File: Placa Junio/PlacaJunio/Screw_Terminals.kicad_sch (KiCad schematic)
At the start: 16 parts, among them J3 Terminal Paracaidas 2, J4 Terminal Paracaidas 1, J5 Terminal Paracaidas 3, J6 Terminal Paracaidas 4, Q2 IRLML0030, Q3 IRLML0030, Q5 IRLML0030, Q6 IRLML0030

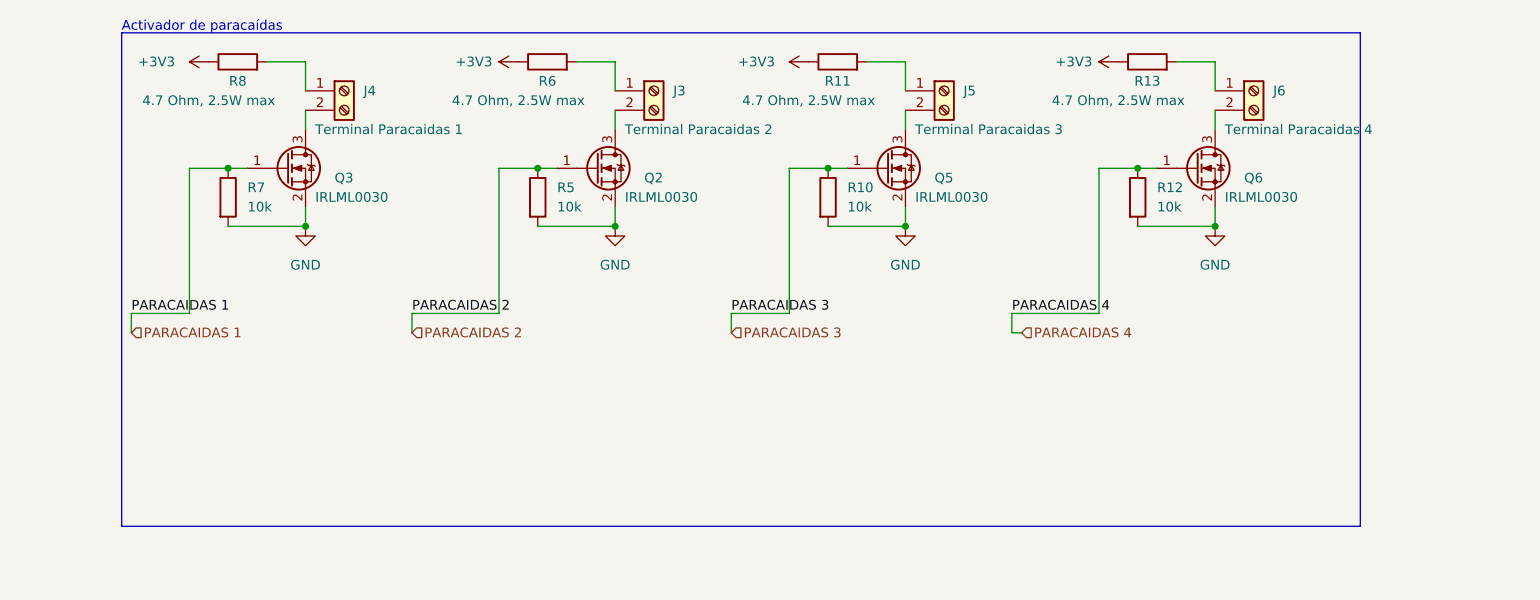
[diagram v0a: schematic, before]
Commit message: Cambios
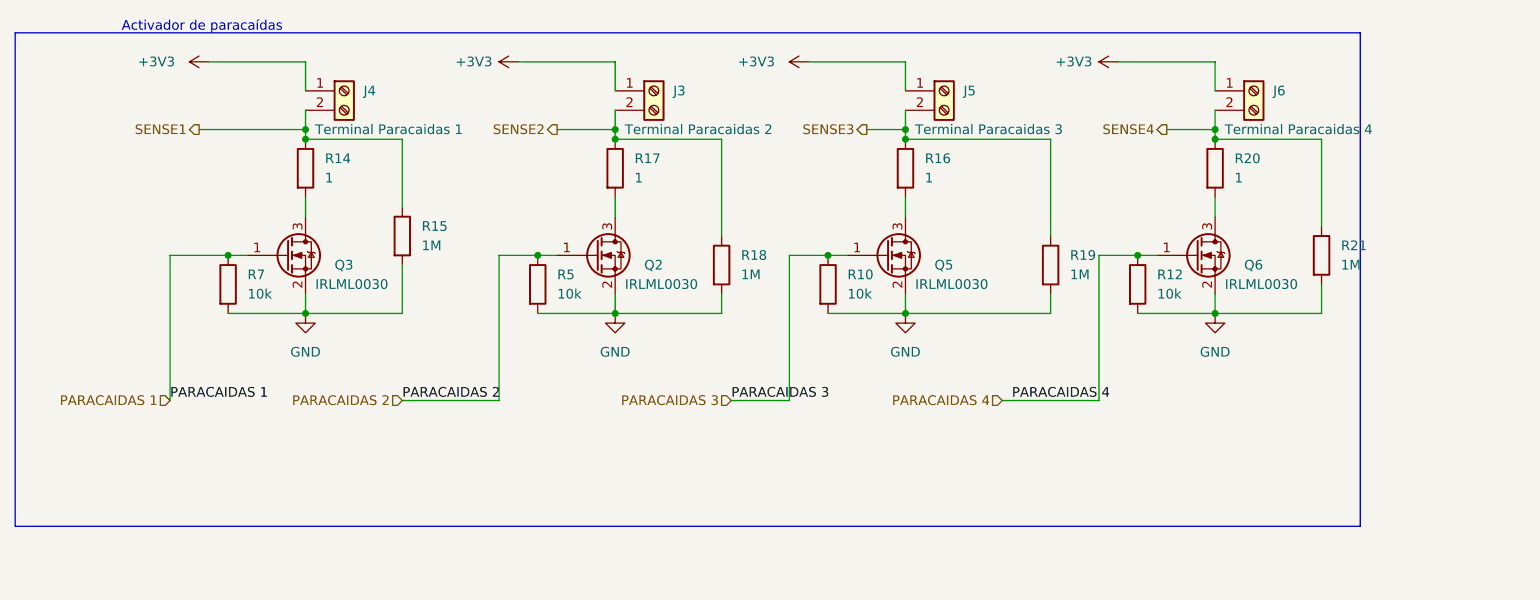
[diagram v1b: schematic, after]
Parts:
- removed R11, R13, R6, R8: 4.7 Ohm, 2.5W max, Resistor_THT:R_Axial_DIN0204_L3.6mm_D1.6mm_P2.54mm_Vertical, symbol Device:R
- added R14, R16, R17, R20: 1, Resistor_SMD:R_0402_1005Metric, symbol Device:R
- added R15, R18, R19, R21: 1M, Resistor_SMD:R_0402_1005Metric, symbol Device:R
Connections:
- net +3V3: now also J3.1 (Pin_1), J4.1 (Pin_1), J5.1 (Pin_1), J6.1 (Pin_1)
- net GND: now also R15.2, R18.2, R19.2, R21.2
- net at Q5.3 (D): now also R16.2; no longer J5.2 (Pin_2)
- net at Q3.3 (D): now also R14.2; no longer J4.2 (Pin_2)
- net at Q2.3 (D): now also R17.2; no longer J3.2 (Pin_2)
- net at Q6.3 (D): now also R20.2; no longer J6.2 (Pin_2)
- new net SENSE1: J4.2 (Pin_2), R14.1, R15.1
- new net SENSE2: J3.2 (Pin_2), R17.1, R18.1
- new net SENSE3: J5.2 (Pin_2), R16.1, R19.1
- new net SENSE4: J6.2 (Pin_2), R20.1, R21.1
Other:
- moved on the sheet: Q2, Q3, Q5, Q6, R10, R12, R5, R7

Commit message: Update Screw_Terminals.kicad_sch
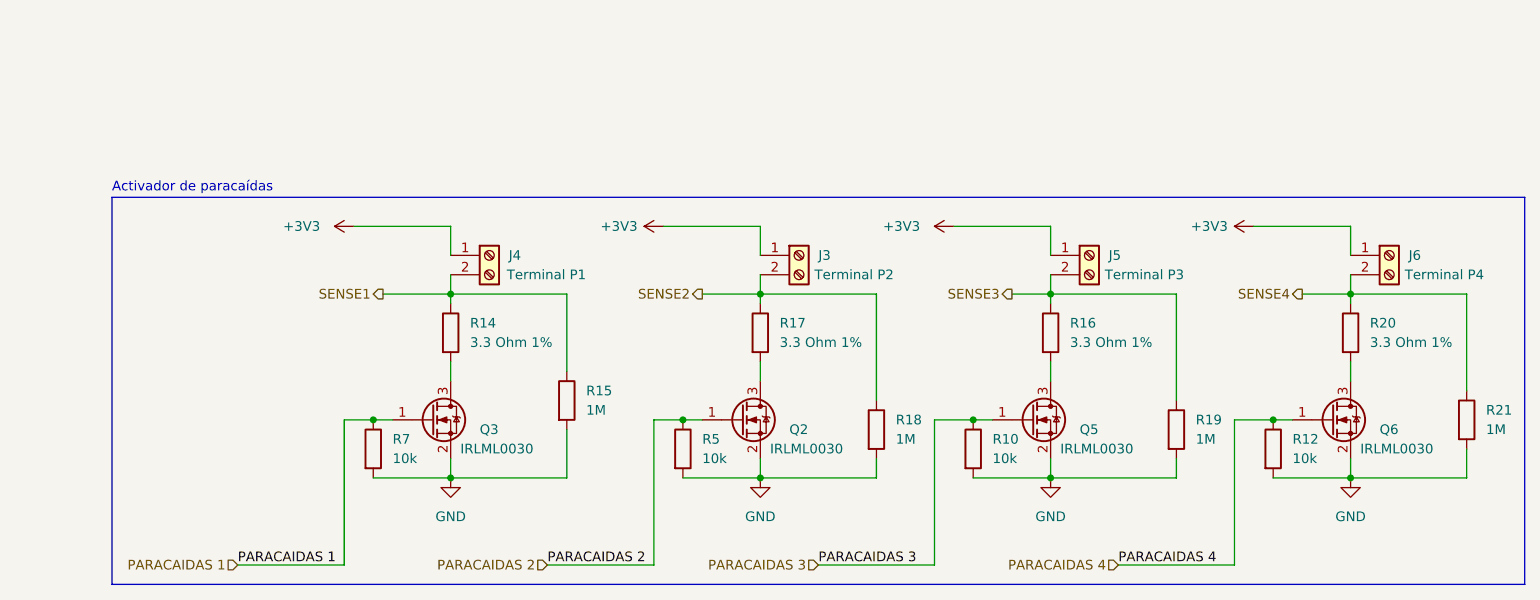
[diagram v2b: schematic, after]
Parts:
- J3: value Terminal Paracaidas 2 -> Terminal P2
- J4: value Terminal Paracaidas 1 -> Terminal P1
- J5: value Terminal Paracaidas 3 -> Terminal P3
- J6: value Terminal Paracaidas 4 -> Terminal P4
- R14, R16, R17, R20: value 1 -> 3.3 Ohm 1%; footprint Resistor_SMD:R_0402_1005Metric -> Resistor_SMD:R_0805_2012Metric; Nº Componente (none) -> RCS08053R30FKEA
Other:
- moved on the sheet: J3, J4, J5, J6, Q2, Q3, Q5, Q6, R10, R12, R14, R15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
